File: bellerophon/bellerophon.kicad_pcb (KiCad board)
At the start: 4 copper layers, 109.6 x 98 mm, 90 parts, among them Q1 ST3413A, Q2 IRLL014NPBF, Q3 IRLL014NPBF, U1 HT7350-A, U2 BNO055, U3 MPL3115A2, U4 Teensy4.0, U5 XTSD, Y1 32.768kHz

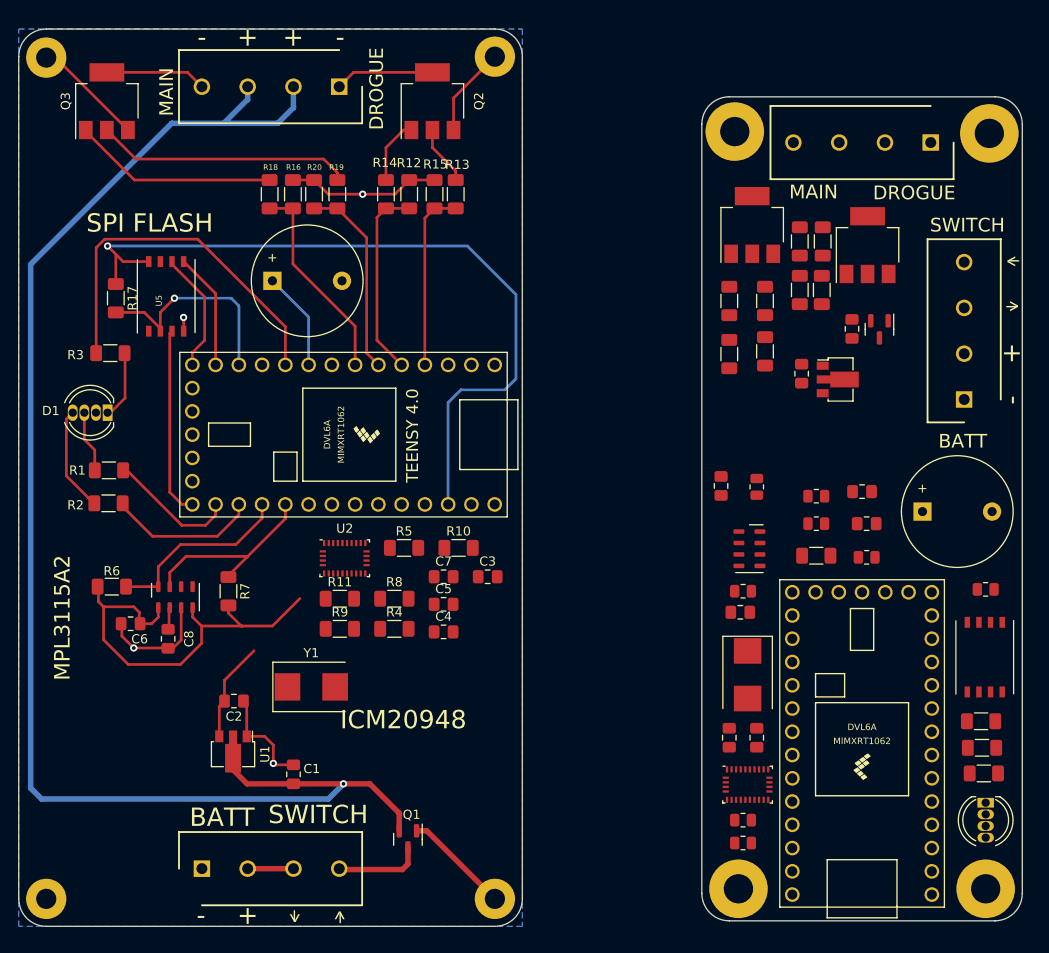
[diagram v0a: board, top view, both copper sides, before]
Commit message: add step file and remove old version of board
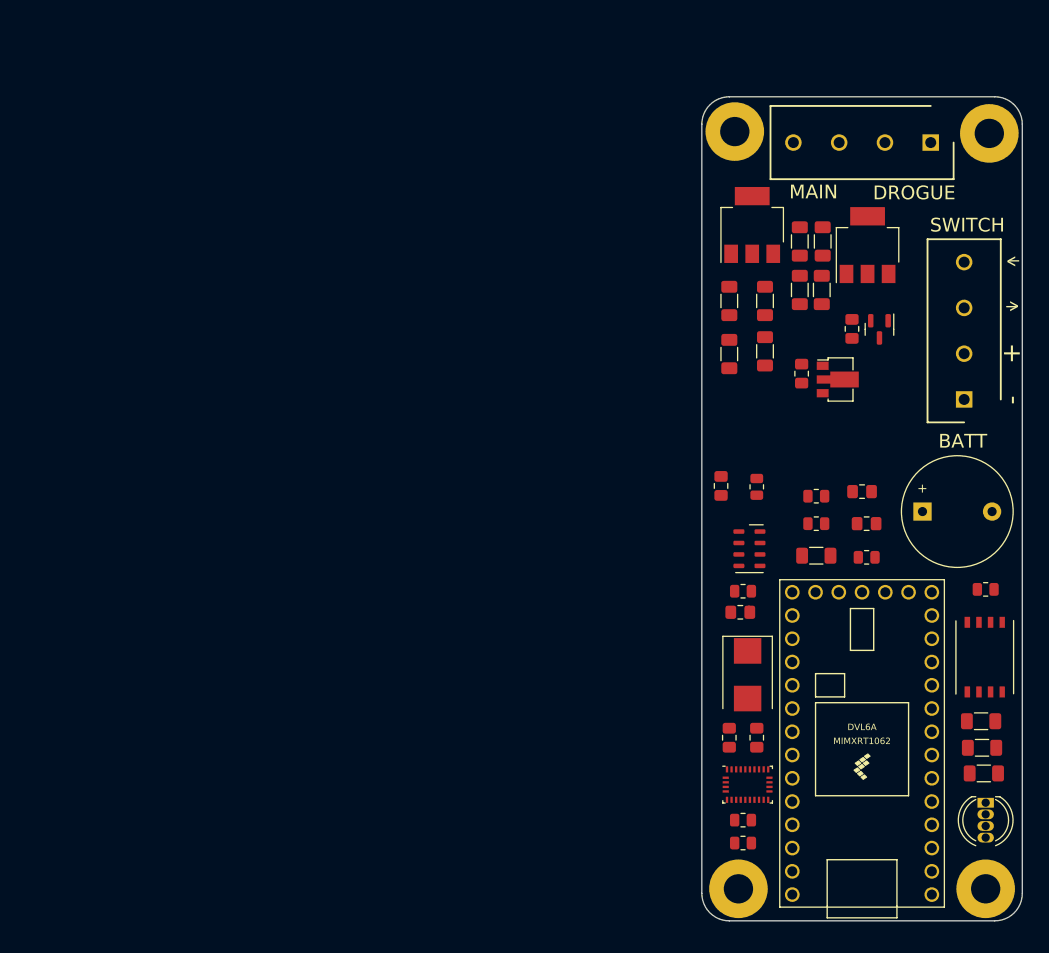
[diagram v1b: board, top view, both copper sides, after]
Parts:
- removed the BZ1 at (155.6, 80.1)
- removed the C1 at (157.9, 134.0)
- removed the C2 at (151.4, 126.0)
- removed the C3 at (179.1, 112.4)
- removed the C4 at (174.3, 118.4)
- removed the C5 at (174.3, 115.4)
- removed the C6 at (140.1, 117.5)
- removed the C7 at (174.3, 112.4)
- removed the C8 at (144.2, 119.2)
- removed the D1 at (137.6, 94.5)
- removed the H1 at (130.9, 147.6)
- removed the H2 at (179.9, 147.6)
- removed the H3 at (130.9, 55.7)
- removed the H4 at (179.9, 55.6)
- removed the PYRO1 at (162.9, 58.9)
- removed the Q1 at (170.4, 141.1)
- removed the Q2 at (173.1, 60.5)
- removed the Q3 at (137.5, 60.5)
- removed the R1 at (137.8, 100.8)
- removed the R10 at (175.9, 109.3)
- removed the R11 at (163.0, 114.8)
- removed the R12 at (170.5, 70.6)
- removed the R13 at (173.3, 70.6)
- removed the R14 at (168.0, 70.6)
- removed the R15 at (175.6, 70.6)
- removed the R16 at (157.8, 70.6)
- removed the R17 at (138.5, 82.0)
- removed the R18 at (155.3, 70.6)
- removed the R19 at (162.7, 70.6)
- removed the R2 at (137.7, 104.4)
- removed the R20 at (160.2, 70.6)
- removed the R3 at (137.9, 88.0)
- removed the R4 at (168.9, 118.1)
- removed the R5 at (170.0, 109.3)
- removed the R6 at (138.1, 113.5)
- removed the R7 at (150.8, 114.0)
- removed the R8 at (168.9, 114.8)
- removed the R9 at (163.0, 118.1)
- removed the TERMINAL1 at (147.9, 144.3)
- removed the U1 at (151.3, 131.5)
- removed the U2 at (163.5, 110.4)
- removed the U3 at (145.0, 114.7)
- removed the U4 at (163.4, 96.9)
- removed the U5 at (144.0, 81.8)
- removed the Y1 at (159.8, 124.5)
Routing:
- net BATT+: track 164.3 -> 0.00 mm, vias 1 -> 0
- net +3.3V: track 131.0 -> 0.00 mm, vias 1 -> 0
- net GND: track 76.4 -> 0.60 mm, vias 4 -> 0
- net RGB3: track 40.7 -> 0.00 mm
- net Net-(PYRO1-Pad4): track 38.9 -> 0.00 mm
- net /CS: track 24.2 -> 0.00 mm, vias 1 -> 0
- net PY2: track 22.4 -> 0.00 mm
- net Net-(Q3-Pad1): track 22.4 -> 0.00 mm
- net PY2_TEST: track 21.5 -> 0.00 mm
- net /SDA1: track 21.3 -> 0.00 mm
- net PY1: track 21.2 -> 0.00 mm
- net /SCL1: track 20.8 -> 0.00 mm
- net /SCK: track 20.7 -> 0.00 mm
- net PY1_TEST: track 19.8 -> 0.00 mm
- net Net-(PYRO1-Pad1): track 17.3 -> 0.00 mm
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- removed copper zone on B.Cu, net GND
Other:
- board size 109.6 x 98 mm -> 35 x 90 mm
- board text removed: "Bellerophon"
- board text removed: "Flight Computer"
- board text removed: "ICM20948"
- board text removed: "MPL3115A2"
- board text removed: "SPI FLASH"
- board text removed: "TEENSY 4.0"
- board text removed: "UNSW ROCKETRY"
